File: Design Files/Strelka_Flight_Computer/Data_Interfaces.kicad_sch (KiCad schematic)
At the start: 9 parts, among them J2 Conn_01x04, J5 USB_B_Micro, J6 USB_B_Micro, U7 USBLC6-2SC6, U8 USBLC6-2SC6, U9 CP2102N-Axx-xQFN28

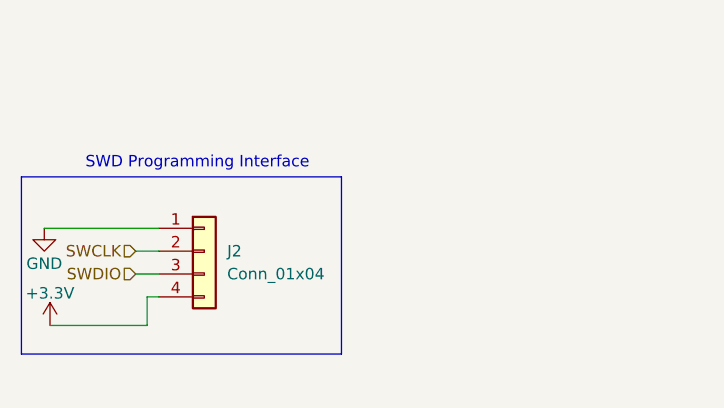
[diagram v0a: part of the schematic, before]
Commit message: Creating BOM
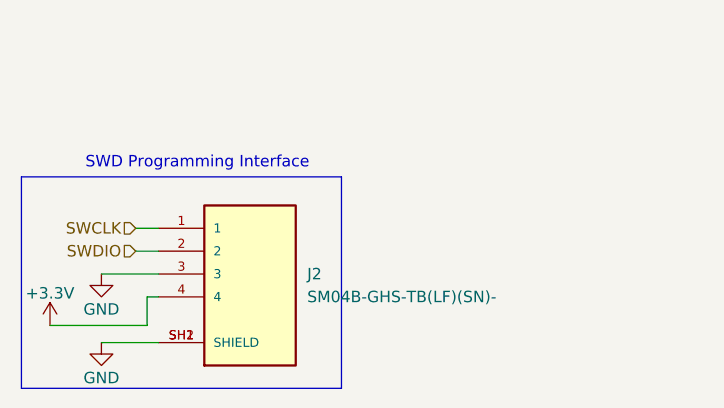
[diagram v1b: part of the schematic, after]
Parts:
- removed J2: Conn_01x04, Connector_PinHeader_2.54mm:PinHeader_1x04_P2.54mm_Horizontal, symbol Connector_Generic:Conn_01x04
- added J2: SM04B-GHS-TB(LF)(SN)-, Footprints:JST_SM04B-GHS-TB(LF)(SN)-, symbol SM04B-GHS-TB_LF__SN_-:SM04B-GHS-TB(LF)(SN)-
- U7, U8: LCSC# (none) -> C2687116
- U9: LCSC# (none) -> C1550553
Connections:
- net +3V3: now also J2.4
- net GND: now also J2.3, J2.SH1 (SHIELD), J2.SH2 (SHIELD)
- net SWCLK: now also J2.1
- net SWDIO: now also J2.2
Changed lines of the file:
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@@
     (stroke (width 0) (type default) (color 0 0 0 0))
   )
-  (polyline (pts (xy 68.58 111.125) (xy 68.58 130.81))
+  (polyline (pts (xy 68.58 111.125) (xy 68.58 134.62))
     (stroke (width 0) (type default) (color 0 0 0 0))
   )
@@
     (stroke (width 0) (type default) (color 0 0 0 0))
   )
-  (wire (pts (xy 81.28 121.92) (xy 83.82 121.92))
+  (wire (pts (xy 77.47 121.92) (xy 83.82 121.92))
     (stroke (width 0) (type default) (color 0 0 0 0))
   )
@@
     (stroke (width 0) (type default) (color 0 0 0 0))
   )
-  (polyline (pts (xy 104.14 130.81) (xy 68.58 130.81))
+  (polyline (pts (xy 104.14 134.62) (xy 68.58 134.62))
     (stroke (width 0) (type default) (color 0 0 0 0))
   )
@@
     (stroke (width 0) (type default) (color 0 0 0 0))
   )
+  (wire (pts (xy 77.47 129.54) (xy 83.82 129.54))
+    (stroke (width 0) (type default) (color 0 0 0 0))
+  )
   (wire (pts (xy 212.09 30.48) (xy 222.885 30.48))
     (stroke (width 0) (type default) (color 0 0 0 0))
@@
     (stroke (width 0) (type default) (color 0 0 0 0))
   )
-  (wire (pts (xy 71.12 116.84) (xy 83.82 116.84))
-    (stroke (width 0) (type default) (color 0 0 0 0))
-  )
   (wire (pts (xy 187.96 85.09) (xy 187.96 97.79))
     (stroke (width 0) (type default) (color 0 0 0 0))
@@
     (stroke (width 0) (type default) (color 0 0 0 0))
   )
-  (polyline (pts (xy 104.14 111.125) (xy 104.14 130.81))
+  (polyline (pts (xy 104.14 111.125) (xy 104.14 134.62))
     (stroke (width 0) (type default) (color 0 0 0 0))
   )
@@
   )
   (wire (pts (xy 194.945 52.07) (xy 212.725 52.07))
+    (stroke (width 0) (type default) (color 0 0 0 0))
+  )
+  (wire (pts (xy 81.28 116.84) (xy 83.82 116.84))
     (stroke (width 0) (type default) (color 0 0 0 0))
   )
@@
     (effects (font (size 1.27 1.27)) (justify left bottom))
   )
-  (hierarchical_label "SWCLK" (shape input) (at 81.28 119.38 180)
+  (hierarchical_label "SWCLK" (shape input) (at 81.28 116.84 180)
     (effects (font (size 1.27 1.27)) (justify right))
   )
-  (hierarchical_label "SWDIO" (shape input) (at 81.28 121.92 180)
+  (hierarchical_label "SWDIO" (shape input) (at 81.28 119.38 180)
     (effects (font (size 1.27 1.27)) (justify right))
   )
@@
       (effects (font (size 1.27 1.27)) hide)
     )
+    (property "LCSC#" "C2687116" (id 4) (at 177.8 55.88 90)
+      (effects (font (size 1.27 1.27)) hide)
+    )
     (pin "1")
     (pin "2")
@@
     (pin "6")
   )
-  (symbol (lib_id "power:GND") (at 71.12 116.84 0) (unit 1)
+  (symbol (lib_id "power:GND") (at 77.47 121.92 0) (unit 1)
     (in_bom yes) (on_board yes)
-    (property "Reference" "#PWR0156" (id 0) (at 71.12 123.19 0)
-      (effects (font (size 1.27 1.27)) hide)
-    )
-    (property "Value" "GND" (id 1) (at 71.12 120.7676 0))
-    (property "Footprint" "" (id 2) (at 71.12 116.84 0)
-      (effects (font (size 1.27 1.27)) hide)
-    )
-    (property "Datasheet" "" (id 3) (at 71.12 116.84 0)
+    (property "Reference" "#PWR0156" (id 0) (at 77.47 128.27 0)
+      (effects (font (size 1.27 1.27)) hide)
+    )
+    (property "Value" "GND" (id 1) (at 77.47 125.8476 0))
+    (property "Footprint" "" (id 2) (at 77.47 121.92 0)
+      (effects (font (size 1.27 1.27)) hide)
+    )
+    (property "Datasheet" "" (id 3) (at 77.47 121.92 0)
       (effects (font (size 1.27 1.27)) hide)
     )
@@
     )
     (property "Datasheet" "" (id 3) (at 167.64 100.33 0)
+      (effects (font (size 1.27 1.27)) hide)
+    )
+    (pin "1")
+  )
+  (symbol (lib_id "power:GND") (at 77.47 129.54 0) (unit 1)
+    (in_bom yes) (on_board yes)
+    (property "Reference" "#PWR0112" (id 0) (at 77.47 135.89 0)
+      (effects (font (size 1.27 1.27)) hide)
+    )
+    (property "Value" "GND" (id 1) (at 77.47 133.4676 0))
+    (property "Footprint" "" (id 2) (at 77.47 129.54 0)
+      (effects (font (size 1.27 1.27)) hide)
+    )
+    (property "Datasheet" "" (id 3) (at 77.47 129.54 0)
       (effects (font (size 1.27 1.27)) hide)
     )
@@
       (effects (font (size 1.27 1.27)) hide)
     )
+    (property "LCSC#" "C2687116" (id 4) (at 177.8 97.79 90)
+      (effects (font (size 1.27 1.27)) hide)
+    )
     (pin "1")
     (pin "2")
@@
     (pin "6")
   )
-  (symbol (lib_id "Connector_Generic:Conn_01x04") (at 88.9 119.38 0) (unit 1)
-    (in_bom yes) (on_board yes) (fields_autoplaced)
-    (property "Reference" "J2" (id 0) (at 91.44 119.3799 0)
-      (effects (font (size 1.27 1.27)) (justify left))
-    )
-    (property "Value" "Conn_01x04" (id 1) (at 91.44 121.9199 0)
-      (effects (font (size 1.27 1.27)) (justify left))
-    )
-    (property "Footprint" "Connector_PinHeader_2.54mm:PinHeader_1x04_P2.54mm_Horizontal" (id 2) (at 88.9 119.38 0)
-      (effects (font (size 1.27 1.27)) hide)
-    )
-    (property "Datasheet" "~" (id 3) (at 88.9 119.38 0)
-      (effects (font (size 1.27 1.27)) hide)
-    )
-    (pin "1")
-    (pin "2")
-    (pin "3")
-    (pin "4")
-  )
   (symbol (lib_id "power:VBUS") (at 160.02 85.09 0) (unit 1)
     (in_bom yes) (on_board yes) (fields_autoplaced)
@@
     (pin "1")
   )
+  (symbol (lib_id "SM04B-GHS-TB_LF__SN_-:SM04B-GHS-TB(LF)(SN)-") (at 93.98 121.92 0) (unit 1)
+    (in_bom yes) (on_board yes) (fields_autoplaced)
+    (property "Reference" "J2" (id 0) (at 100.33 121.9199 0)
+      (effects (font (size 1.27 1.27)) (justify left))
+    )
+    (property "Value" "SM04B-GHS-TB(LF)(SN)-" (id 1) (at 100.33 124.4599 0)
+      (effects (font (size 1.27 1.27)) (justify left))
+    )
+    (property "Footprint" "Footprints:JST_SM04B-GHS-TB(LF)(SN)-" (id 2) (at 93.98 121.92 0)
+      (effects (font (size 1.27 1.27)) (justify left bottom) hide)
+    )
+    (property "Datasheet" "https://datasheet.lcsc.com/lcsc/1810261120_JST-Sales-America-SM04B-GHS-TB-LF-SN_C189895.pdf" (id 3) (at 93.98 121.92 0)
+      (effects (font (size 1.27 1.27)) (justify left bottom) hide)
+    )
+    (property "LCSC#" "C189895" (id 4) (at 93.98 121.92 0)
+      (effects (font (size 1.27 1.27)) hide)
+    )
+    (pin "1")
+    (pin "2")
+    (pin "3")
+    (pin "4")
+    (pin "SH1")
+    (pin "SH2")
+  )
   (symbol (lib_id "power:GND") (at 225.425 100.33 0) (unit 1)
     (in_bom yes) (on_board yes) (fields_autoplaced)
@@
       (effects (font (size 1.27 1.27)) hide)
     )
+    (property "LCSC#" "C1550553" (id 4) (at 225.425 67.31 0)
+      (effects (font (size 1.27 1.27)) hide)
+    )
